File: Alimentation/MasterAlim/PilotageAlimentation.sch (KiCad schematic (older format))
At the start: 7 parts, among them J4 INHIBIT, J5 ToRegul, U1 74LVC1G02

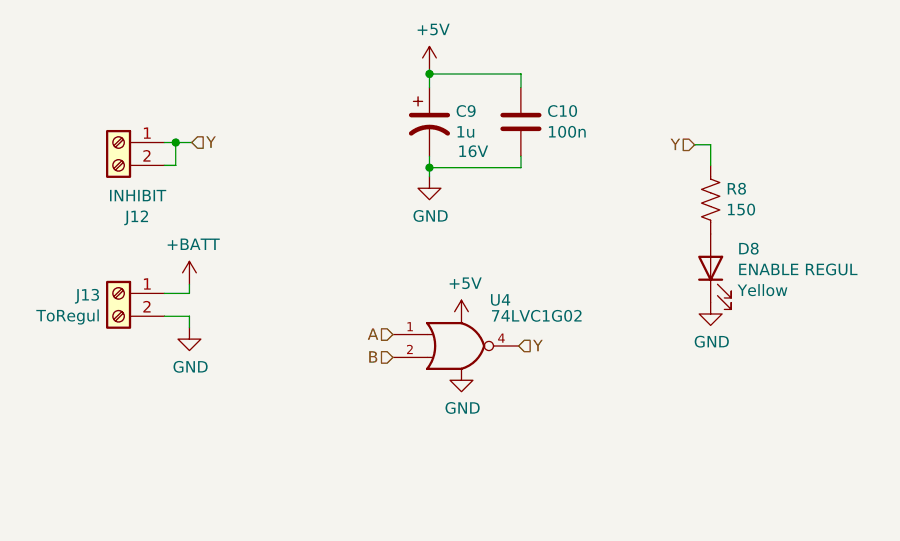
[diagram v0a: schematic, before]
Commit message: Finalisation alimentations
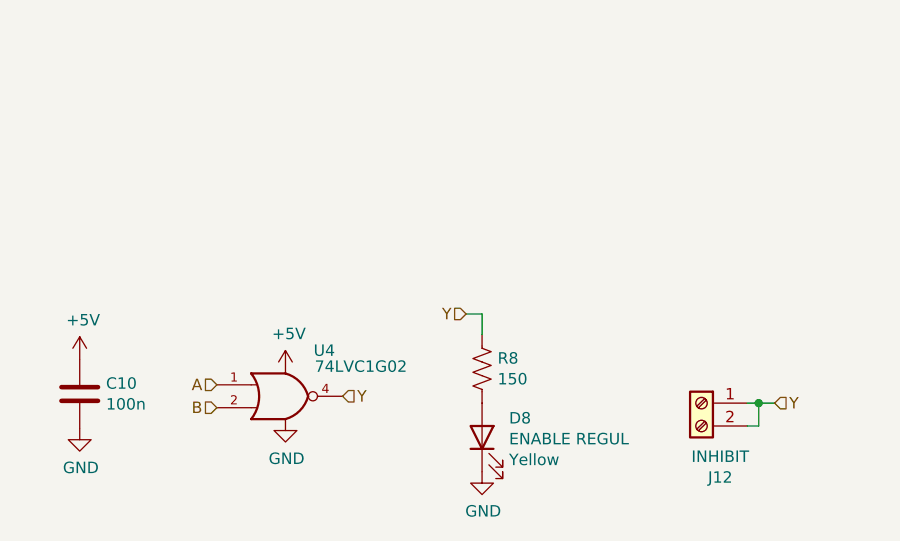
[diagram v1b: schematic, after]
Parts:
- removed C1: 1u, Capacitor_SMD:CP_Elec_4x5.3, symbol Device:CP1
- removed J5: ToRegul, TerminalBlock_Phoenix:TerminalBlock_Phoenix_MKDS-1,5-2-5.08_1x02_P5.08mm_Horizontal, symbol Connector:Screw_Terminal_01x02
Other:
- moved on the sheet: C10, D8, J12, R8, U4
